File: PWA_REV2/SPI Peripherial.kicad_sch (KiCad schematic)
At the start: 33 parts, among them J401 RJ12_6P6C_HORZ, Q302 BSS138, Q303 BSS138, Q304 BSS138, Q305 BSS138

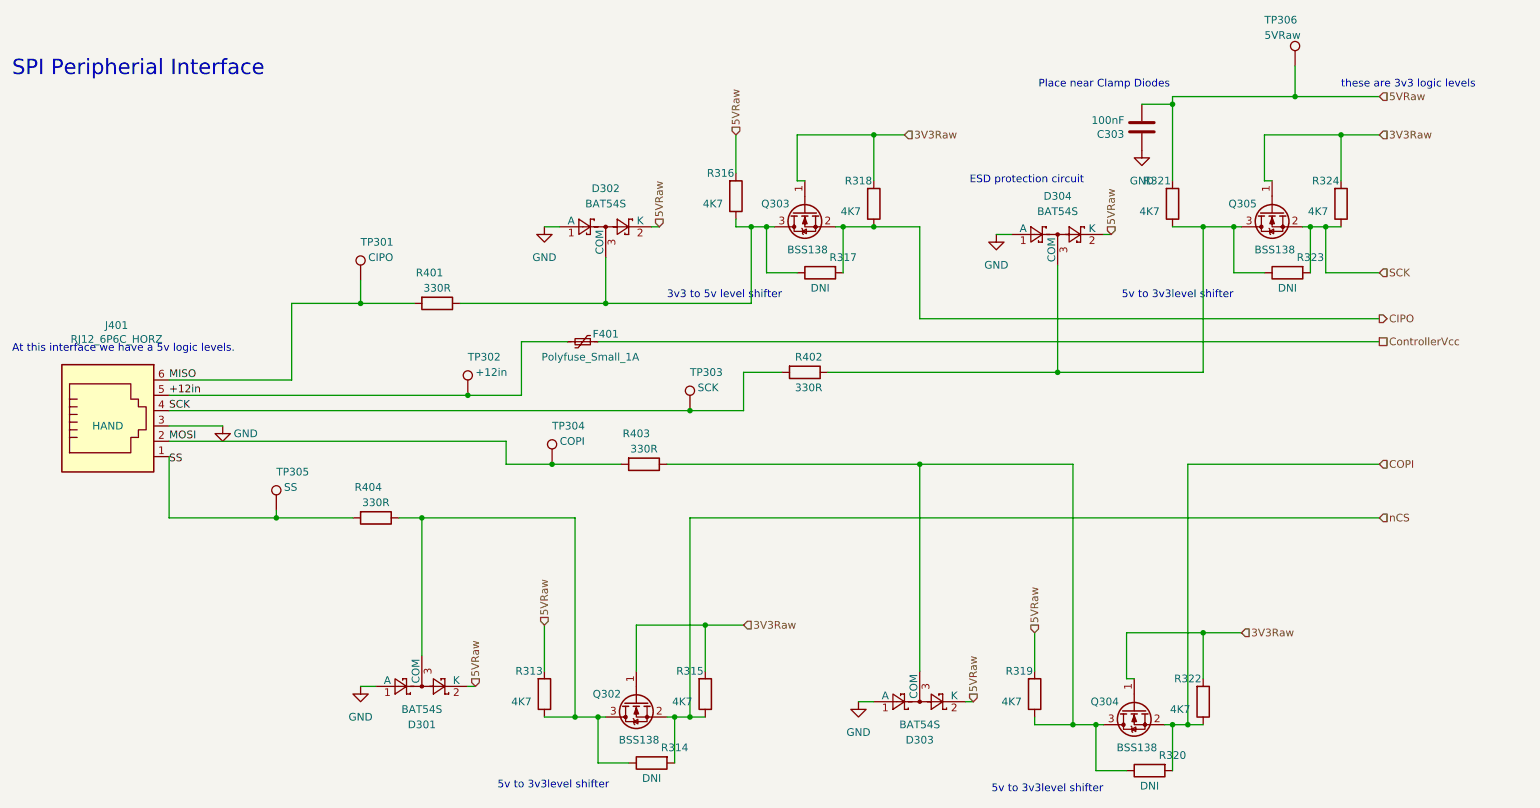
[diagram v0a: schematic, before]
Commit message: Revert "Hardware, PWA, Add a Jumper to BOM for J102 so that USB Connector Can Power Krake, issue 312."
This reverts commit c2819b8ee4999f733f52d823f88f6aefd6456fcc.
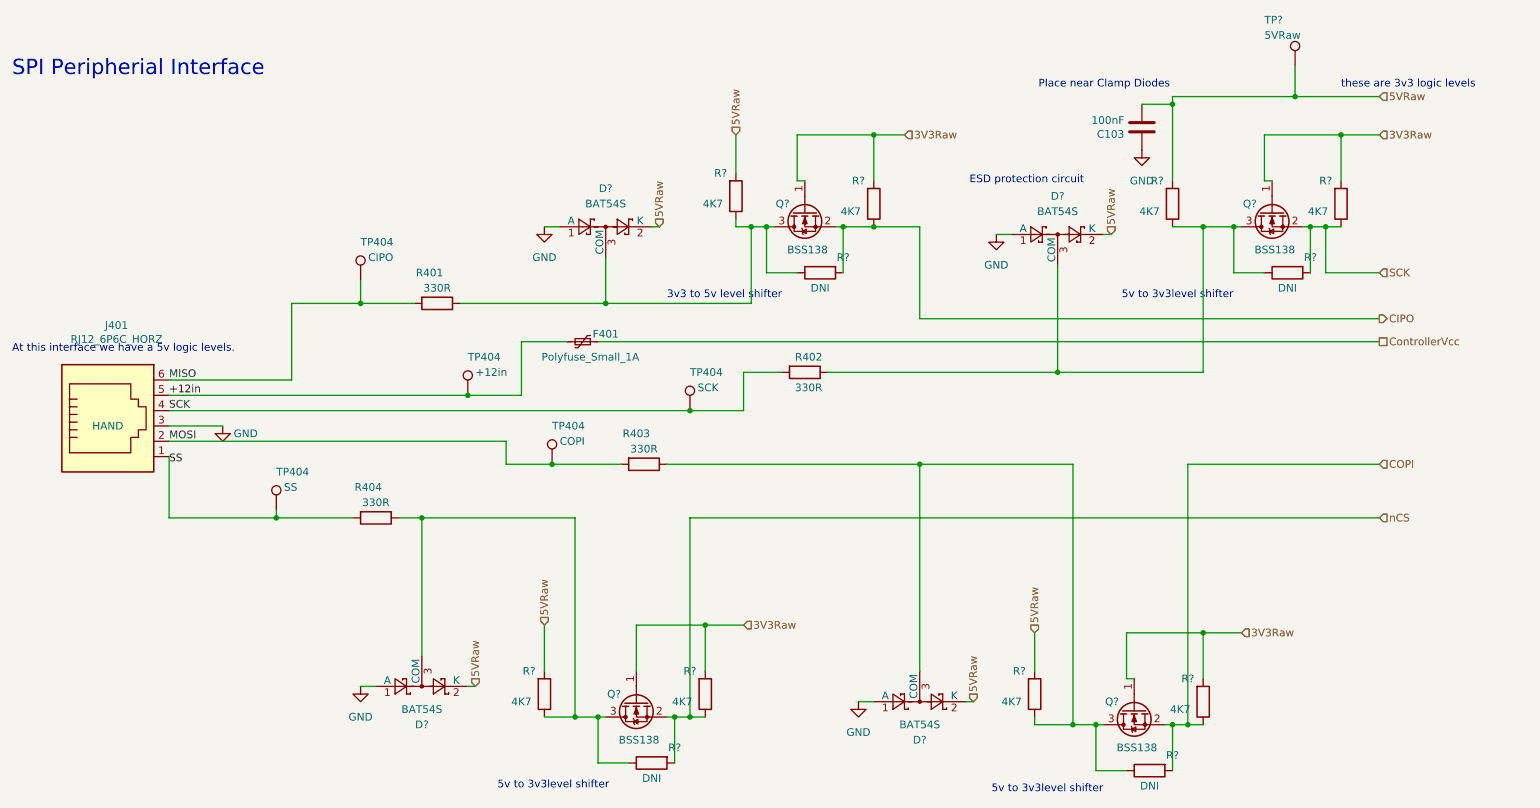
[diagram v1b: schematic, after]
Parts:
- renumbered C303 to C103, D303 to D?, D301 to D?, D302 to D?, D304 to D?, Q305 to Q?, Q302 to Q?, Q303 to Q?, Q304 to Q?, R319 to R?, R320 to R?, R313 to R?, R322 to R?, R315 to R?, R317 to R?, R316 to R?, R321 to R?, R324 to R?, R323 to R?, R318 to R?, R314 to R?, TP302 to TP404, TP301 to TP404, TP303 to TP404, TP304 to TP404, TP305 to TP404, TP306 to TP?
